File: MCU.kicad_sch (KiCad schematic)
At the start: 37 parts, among them J301 SWD, J302 USB_C_Receptacle_USB2.0, SW301 SW_SPDT, U301 STM32F405RGT6, U302 USBLC6-2SC6, Y301 16MHz

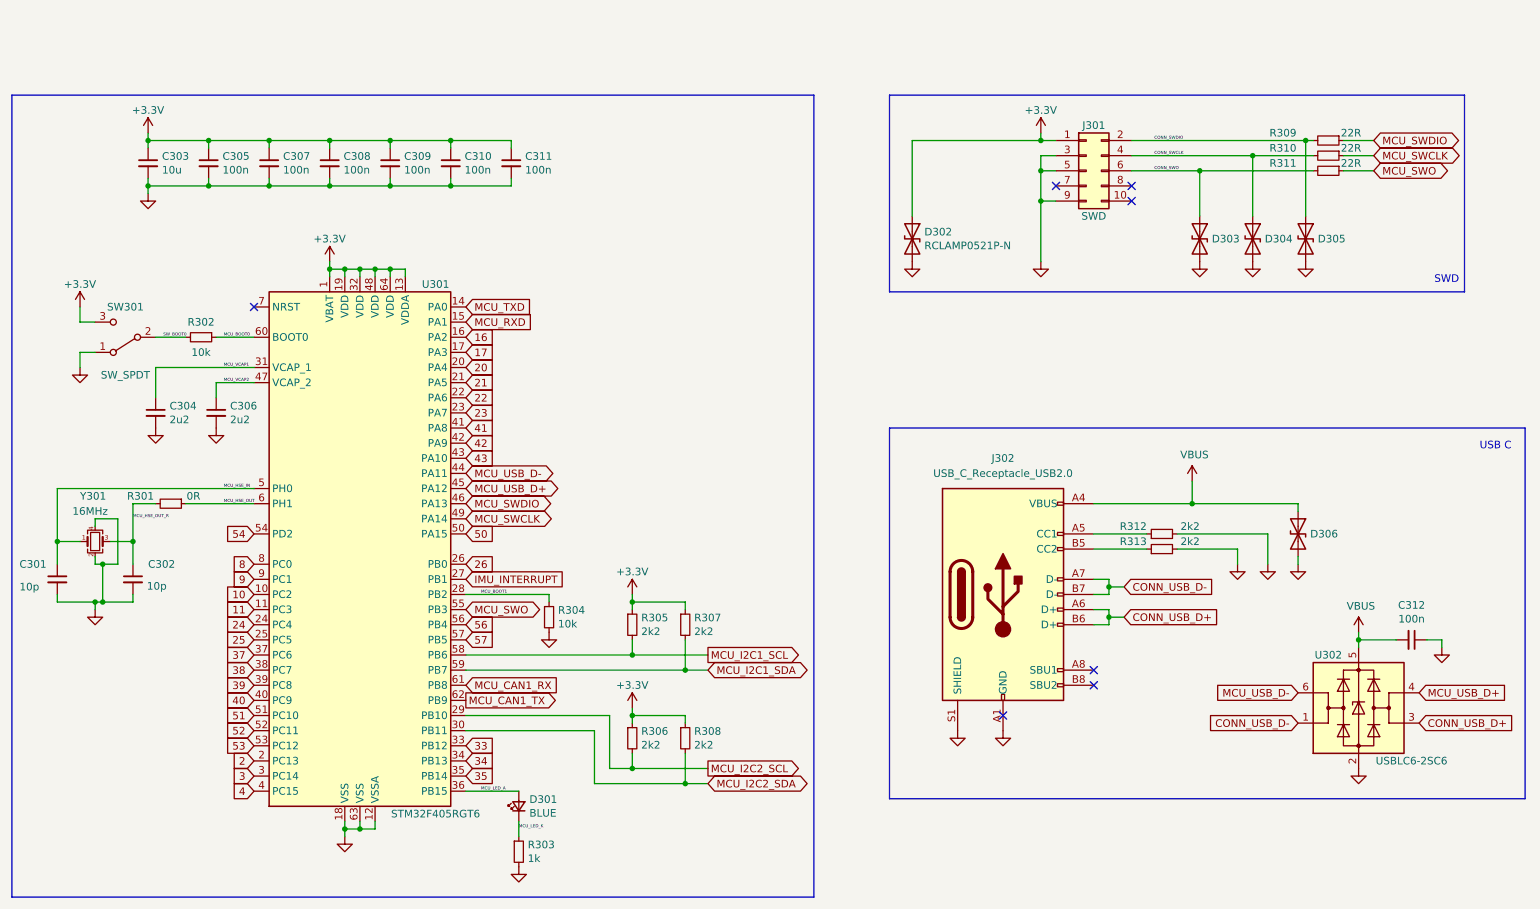
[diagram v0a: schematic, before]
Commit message: final commit before holiday
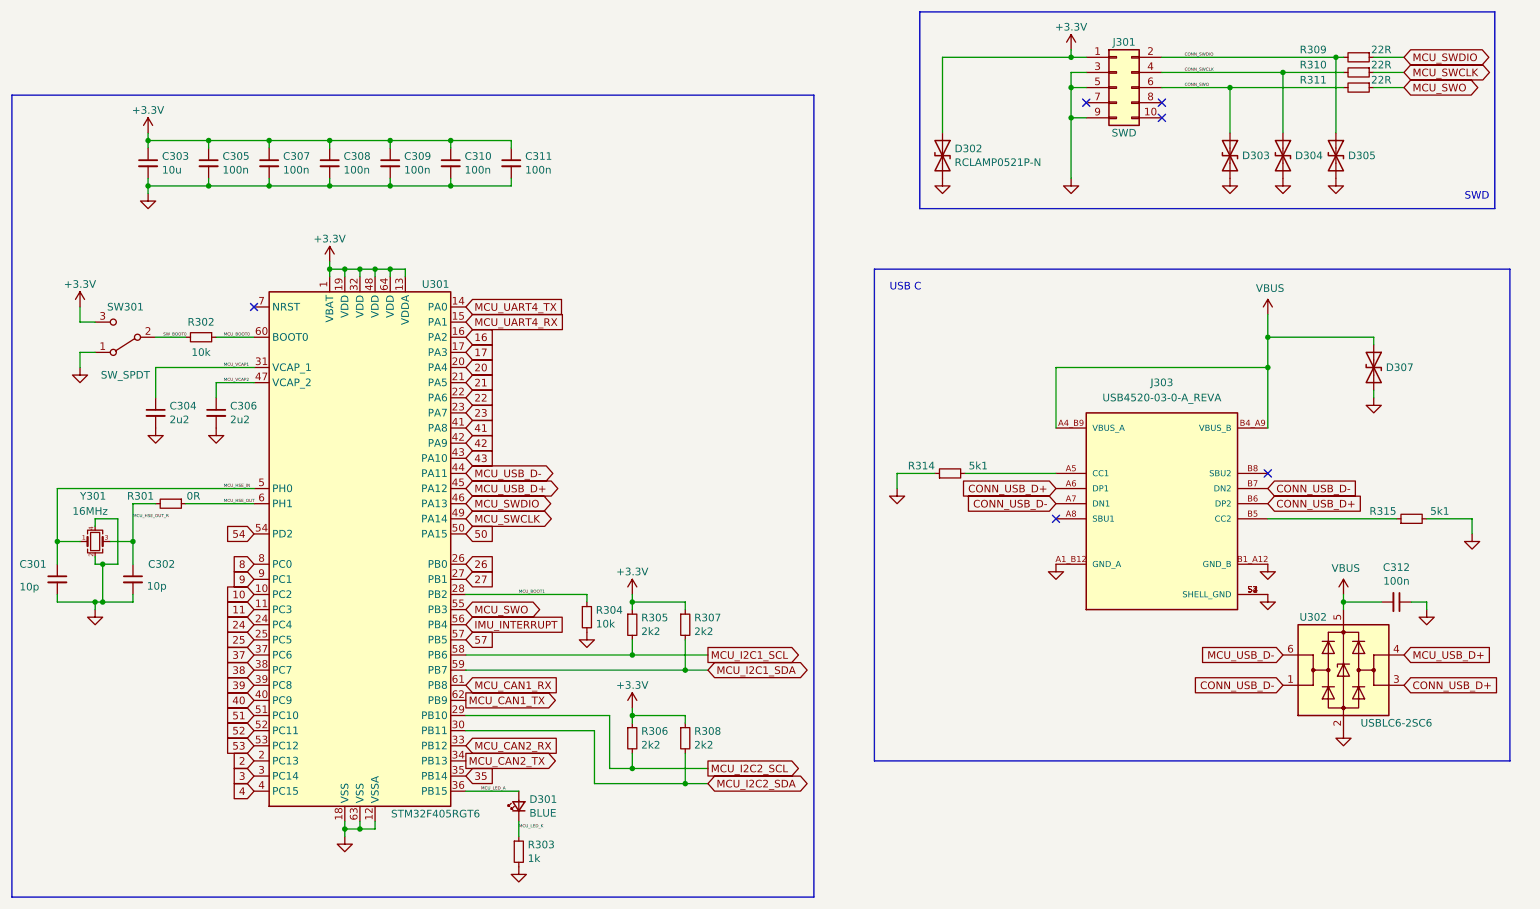
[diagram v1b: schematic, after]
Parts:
- removed D306: RCLAMP0521P-N, Diode_SMD:D_0402_1005Metric, symbol Device:D_TVS
- removed J302: USB_C_Receptacle_USB2.0, Connector_USB:USB_C_Receptacle_XKB_U262-16XN-4BVC11, symbol Connector:USB_C_Receptacle_USB2.0
- removed R312, R313: 2k2, Resistor_SMD:R_0402_1005Metric, symbol Device:R_Small
- added D307: RCLAMP0521P-N, Diode_SMD:D_0402_1005Metric, symbol Device:D_TVS
- added J303: USB4520-03-0-A_REVA, SnapEDA Library:GCT_USB4520-03-0-A_REVA, symbol USB4520-03-0-A_REVA:USB4520-03-0-A_REVA
- added R314, R315: 5k1, Resistor_SMD:R_0402_1005Metric, symbol Device:R_Small
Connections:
- net 56 is gone; now on net IMU_INTERRUPT: U301.56 (PB4)
- net CONN_USB_D+: now also J303.A6 (DP1), J303.B6 (DP2)
- net CONN_USB_D-: now also J303.A7 (DN1), J303.B7 (DN2)
- net GND: now also D307.2 (A2), J303.A1_B12 (GND_A), J303.B1_A12 (GND_B), J303.S1 (SHELL_GND), J303.S2 (SHELL_GND), J303.S3 (SHELL_GND), J303.S4 (SHELL_GND), R314.1, R315.2
- net IMU_INTERRUPT: no longer U301.27 (PB1)
- net VBUS: now also D307.1 (A1), J303.A4_B9 (VBUS_A), J303.B4_A9 (VBUS_B)
- net 33 renamed MCU_CAN2_RX
- net 34 renamed MCU_CAN2_TX
- net MCU_RXD renamed MCU_UART4_RX
- net MCU_TXD renamed MCU_UART4_TX
- new net: J303.B5 (CC2), R315.1
- new net: J303.A5 (CC1), R314.2
- new net 27: U301.27 (PB1)
- no-connect marks 7 -> 6
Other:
- moved on the sheet: C312, D302, D303, D304, D305, J301, R304, R309, R310, R311, U302
